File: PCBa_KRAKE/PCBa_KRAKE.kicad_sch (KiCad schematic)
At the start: 51 parts, among them J101 Barrel_Jack_Switch_SMT, J102 0.100_2Pin, J103 0.100_2Pin, U1 AMS1117-3.3, U101 LM7805_TO220, U102 ESP32-WROOM-32D

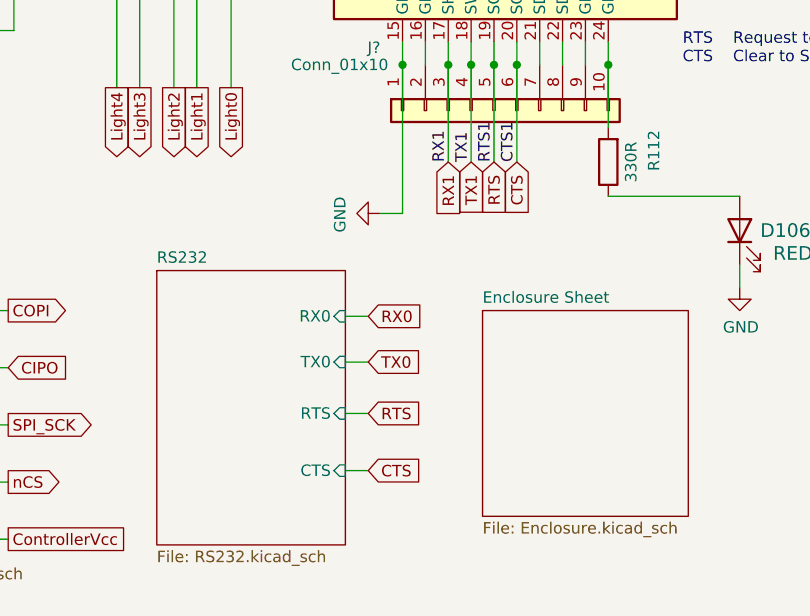
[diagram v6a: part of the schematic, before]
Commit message: Fixing Global label of RS232.
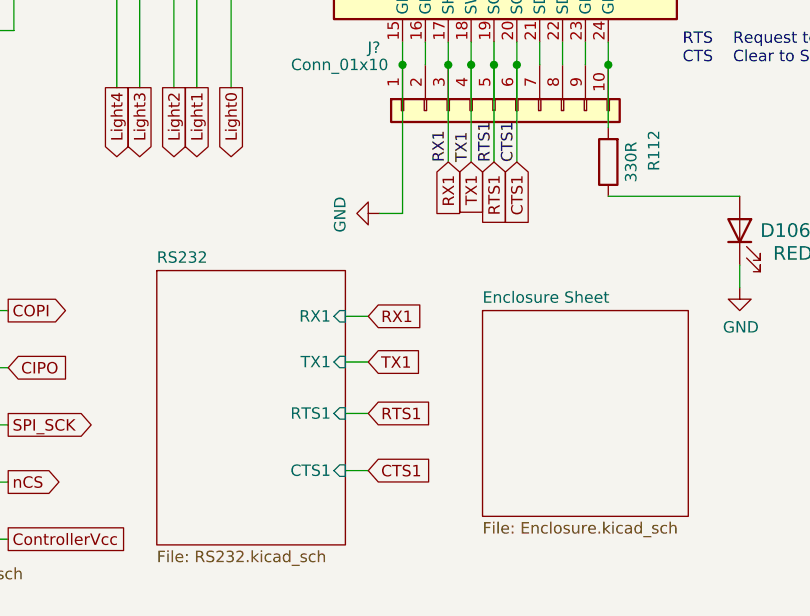
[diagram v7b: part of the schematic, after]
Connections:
- net CTS renamed CTS1
- net RTS renamed RTS1
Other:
- sheet RS232 ports: added CTS1, RTS1, RX1, TX1; removed CTS, RTS, RX0, TX0
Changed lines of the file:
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@@
     )
   )
-  (global_label "TX0" (shape input) (at 132.715 173.355 0) (fields_autoplaced)
-    (effects (font (size 1.27 1.27)) (justify left))
-    (property "Intersheetrefs" "${INTERSHEET_REFS}" (at 138.3532 173.355 0)
-      (effects (font (size 1.27 1.27)) (justify left) hide)
-    )
-  )
   (global_label "Switch_Mute" (shape input) (at 113.665 106.045 180) (fields_autoplaced)
     (effects (font (size 1.27 1.27)) (justify right))
@@
     )
   )
-  (global_label "CTS" (shape input) (at 132.715 185.42 0) (fields_autoplaced)
-    (effects (font (size 1.27 1.27)) (justify left))
-    (property "Intersheetrefs" "${INTERSHEET_REFS}" (at 138.4137 185.42 0)
-      (effects (font (size 1.27 1.27)) (justify left) hide)
-    )
-  )
-  (global_label "RTS" (shape input) (at 146.685 151.13 270) (fields_autoplaced)
+  (global_label "RTS1" (shape input) (at 146.685 151.13 270) (fields_autoplaced)
     (effects (font (size 1.27 1.27)) (justify right))
-    (property "Intersheetrefs" "${INTERSHEET_REFS}" (at 146.685 156.8287 90)
+    (property "Intersheetrefs" "${INTERSHEET_REFS}" (at 146.685 158.0382 90)
       (effects (font (size 1.27 1.27)) (justify right) hide)
     )
@@
     )
   )
+  (global_label "RTS1" (shape input) (at 132.715 179.07 0) (fields_autoplaced)
+    (effects (font (size 1.27 1.27)) (justify left))
+    (property "Intersheetrefs" "${INTERSHEET_REFS}" (at 139.6232 179.07 0)
+      (effects (font (size 1.27 1.27)) (justify left) hide)
+    )
+  )
   (global_label "SPI_SCK" (shape input) (at 202.565 111.125 0) (fields_autoplaced)
     (effects (font (size 1.27 1.27)) (justify left))
@@
     )
   )
+  (global_label "CTS1" (shape input) (at 132.715 185.42 0) (fields_autoplaced)
+    (effects (font (size 1.27 1.27)) (justify left))
+    (property "Intersheetrefs" "${INTERSHEET_REFS}" (at 139.6232 185.42 0)
+      (effects (font (size 1.27 1.27)) (justify left) hide)
+    )
+  )
   (global_label "SPI_SCK" (shape output) (at 92.71 180.34 0) (fields_autoplaced)
     (effects (font (size 1.27 1.27)) (justify left))
@@
     )
   )
+  (global_label "RX1" (shape input) (at 132.715 168.275 0) (fields_autoplaced)
+    (effects (font (size 1.27 1.27)) (justify left))
+    (property "Intersheetrefs" "${INTERSHEET_REFS}" (at 138.6556 168.275 0)
+      (effects (font (size 1.27 1.27)) (justify left) hide)
+    )
+  )
   (global_label "nCS" (shape input) (at 197.485 113.665 0) (fields_autoplaced)
     (effects (font (size 1.27 1.27)) (justify left))
@@
     )
   )
-  (global_label "CTS" (shape input) (at 149.225 151.13 270) (fields_autoplaced)
+  (global_label "CTS1" (shape input) (at 149.225 151.13 270) (fields_autoplaced)
     (effects (font (size 1.27 1.27)) (justify right))
-    (property "Intersheetrefs" "${INTERSHEET_REFS}" (at 149.225 156.8287 90)
+    (property "Intersheetrefs" "${INTERSHEET_REFS}" (at 149.225 158.0382 90)
       (effects (font (size 1.27 1.27)) (justify right) hide)
     )
   )
-  (global_label "RTS" (shape input) (at 132.715 179.07 0) (fields_autoplaced)
-    (effects (font (size 1.27 1.27)) (justify left))
-    (property "Intersheetrefs" "${INTERSHEET_REFS}" (at 138.4137 179.07 0)
-      (effects (font (size 1.27 1.27)) (justify left) hide)
-    )
-  )
   (global_label "COPI" (shape output) (at 92.71 167.64 0) (fields_autoplaced)
     (effects (font (size 1.27 1.27)) (justify left))
@@
     )
   )
+  (global_label "TX1" (shape input) (at 132.715 173.355 0) (fields_autoplaced)
+    (effects (font (size 1.27 1.27)) (justify left))
+    (property "Intersheetrefs" "${INTERSHEET_REFS}" (at 138.3532 173.355 0)
+      (effects (font (size 1.27 1.27)) (justify left) hide)
+    )
+  )
   (global_label "Light0" (shape output) (at 252.095 137.16 180) (fields_autoplaced)
     (effects (font (size 1.27 1.27)) (justify right))
@@
     )
   )
-  (global_label "RX0" (shape input) (at 132.715 168.275 0) (fields_autoplaced)
-    (effects (font (size 1.27 1.27)) (justify left))
-    (property "Intersheetrefs" "${INTERSHEET_REFS}" (at 138.6556 168.275 0)
-      (effects (font (size 1.27 1.27)) (justify left) hide)
-    )
-  )
   (global_label "COPI" (shape input) (at 205.105 93.345 0) (fields_autoplaced)
     (effects (font (size 1.27 1.27)) (justify left))
@@
       (effects (font (size 1.27 1.27)) (justify left top))
     )
-    (pin "RX0" input (at 130.175 168.275 0)
+    (pin "RTS1" input (at 130.175 179.07 0)
       (effects (font (size 1.27 1.27)) (justify right))
     )
-    (pin "TX0" input (at 130.175 173.355 0)
+    (pin "CTS1" input (at 130.175 185.42 0)
       (effects (font (size 1.27 1.27)) (justify right))
     )
-    (pin "CTS" input (at 130.175 185.42 0)
+    (pin "RX1" input (at 130.175 168.275 0)
       (effects (font (size 1.27 1.27)) (justify right))
     )
-    (pin "RTS" input (at 130.175 179.07 0)
+    (pin "TX1" input (at 130.175 173.355 0)
       (effects (font (size 1.27 1.27)) (justify right))
     )
